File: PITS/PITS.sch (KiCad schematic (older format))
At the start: 38 parts, among them P1 CONN_02X20, P14 BATT, P2 BNC, P3 BNC, P4 BNC, P5 BNC, P6 Batt, P7 SENSOR, U1 HX1, U2 MAX-M8C/Q, U3 MTX2, U4 RFM9*, U7 MCP3426, U8 BME280

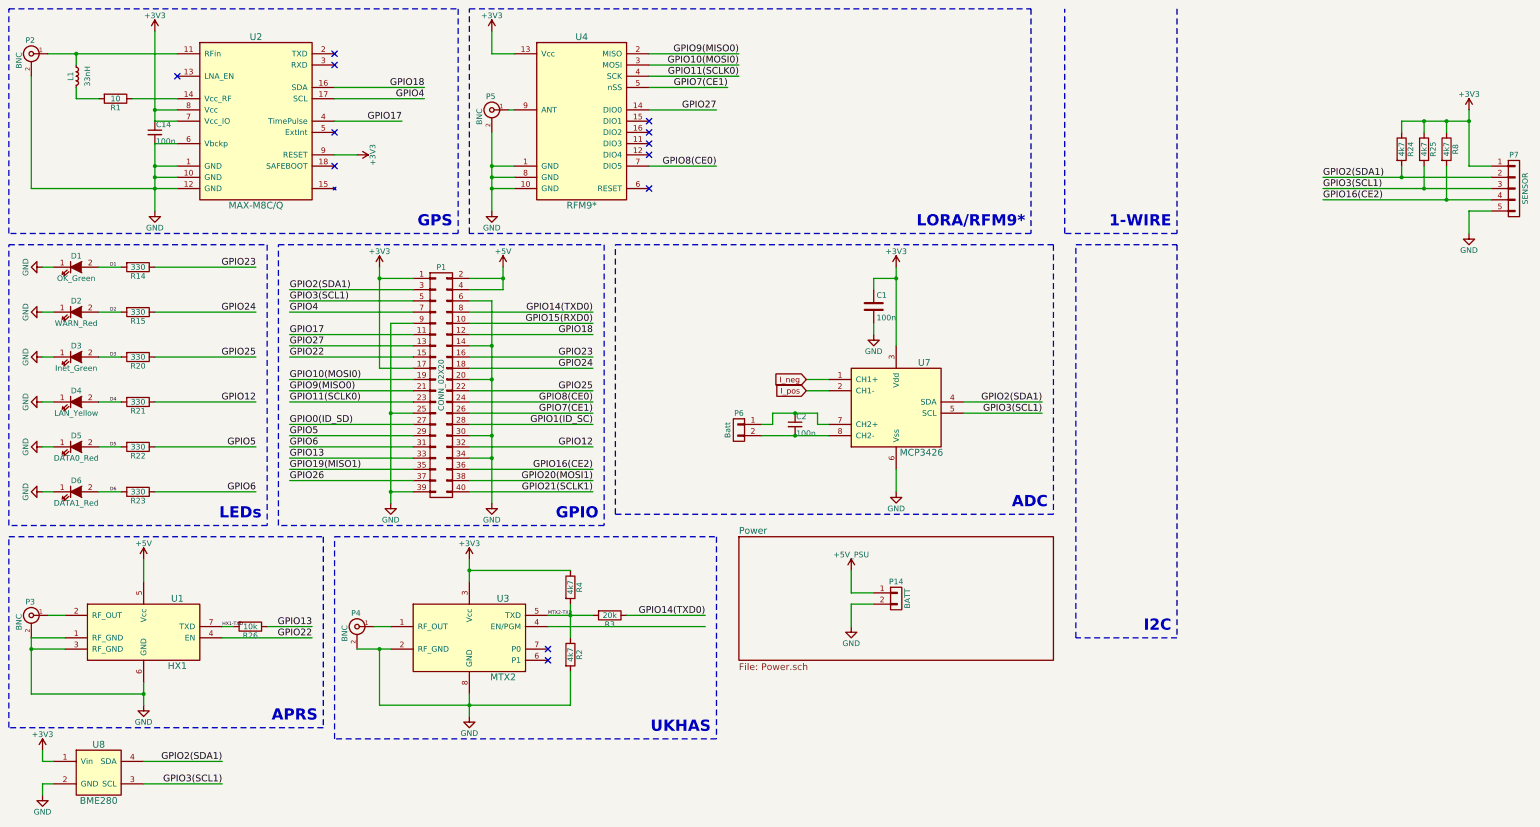
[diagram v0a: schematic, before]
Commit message: Cleand up plan
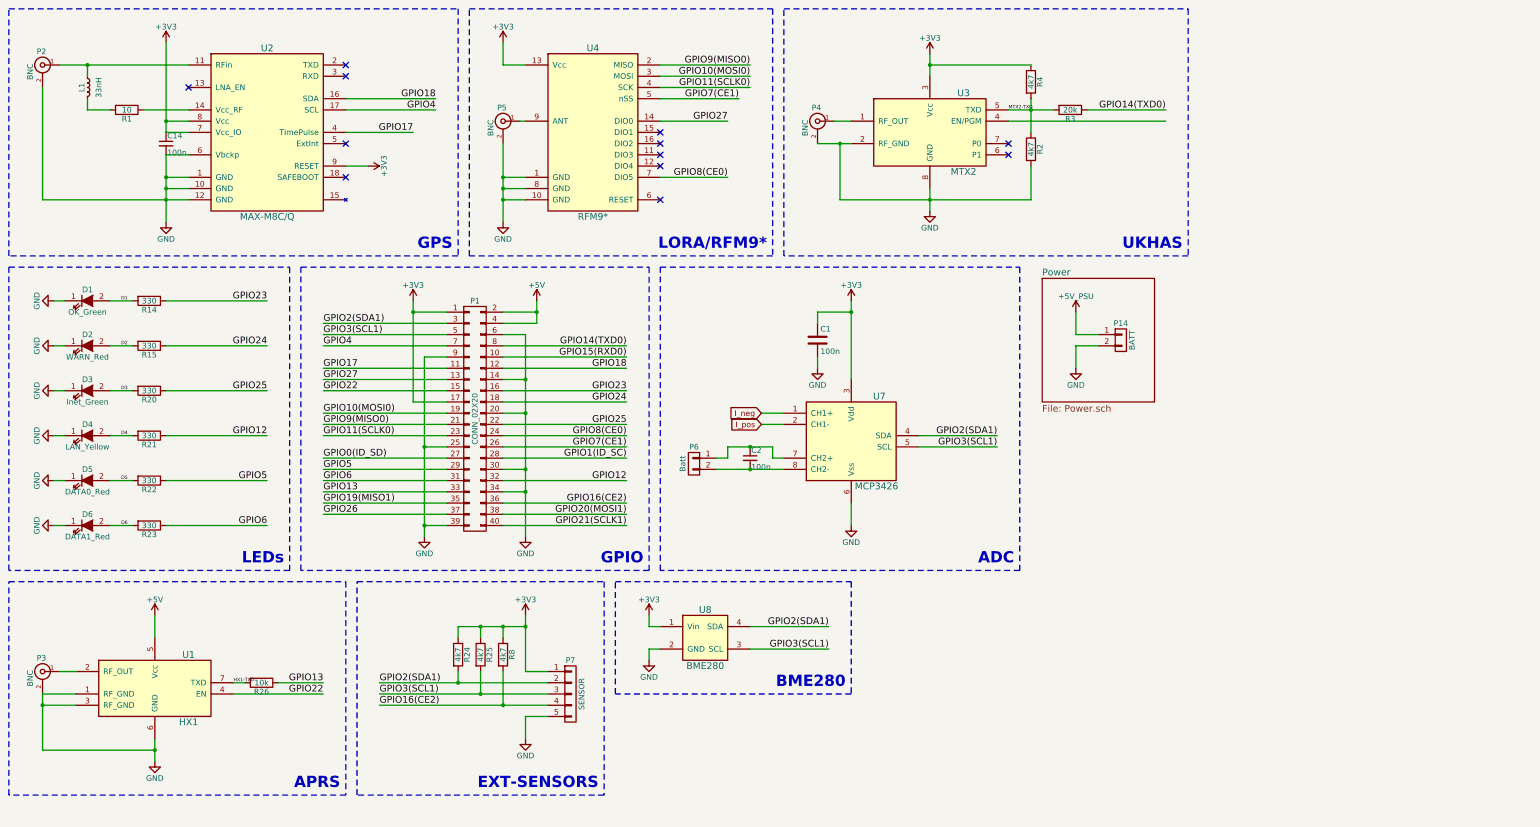
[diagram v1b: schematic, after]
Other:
- note added: "BME280"
- note added: "EXT-SENSORS"
- note removed: "1-WIRE"
- note removed: "I2C"
- moved on the sheet: C1, C14, C2, D1, D2, D3, D4, D5, D6, L1, P1, P14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
